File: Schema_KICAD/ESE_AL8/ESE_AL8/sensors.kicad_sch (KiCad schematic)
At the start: 27 parts, among them J201 JTAG/SWD, J202 Moteur1, J203 Moteur2, J204 LIDAR, J205 CB1, J206 CB2, J207 CB3, J208 CB4, SW201 SW_c/s, U201 ZXBM5210-SP, U202 ZXBM5210-SP, U203 ADXL343

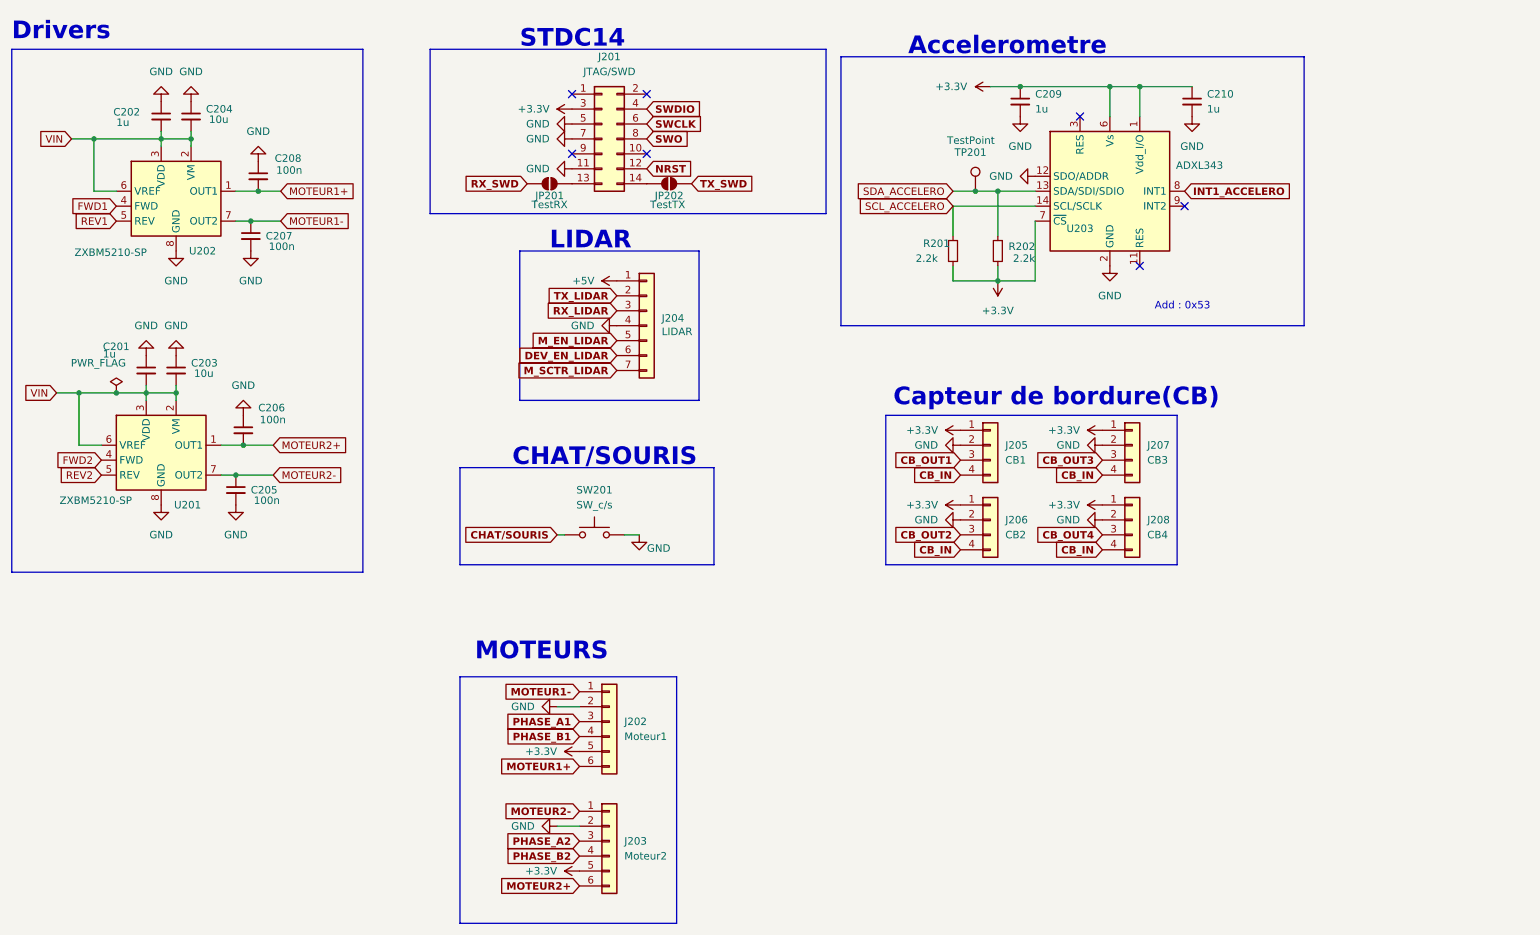
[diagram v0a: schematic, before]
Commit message: commit du code et kicad modifié
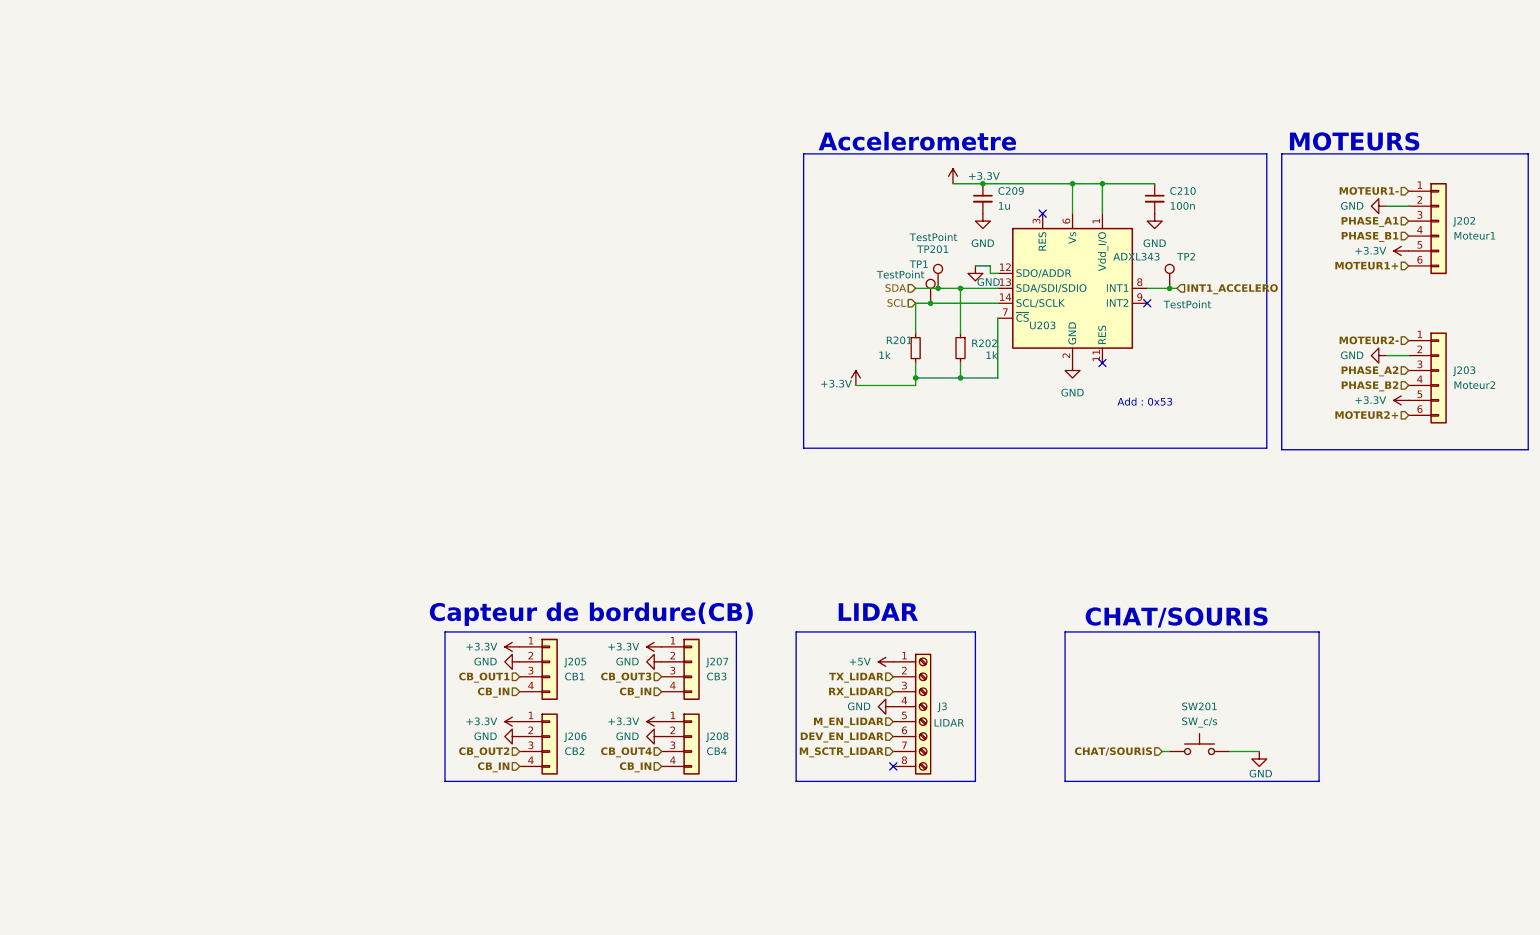
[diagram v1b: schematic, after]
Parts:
- removed C201, C202: 1u, Capacitor_SMD:C_0402_1005Metric_Pad0.74x0.62mm_HandSolder, symbol Device:C_Small
- removed C203, C204: 10u, Capacitor_SMD:C_0603_1608Metric_Pad1.08x0.95mm_HandSolder, symbol Device:C_Small
- removed C205, C206, C207, C208: 100n, Capacitor_SMD:C_0402_1005Metric_Pad0.74x0.62mm_HandSolder, symbol Device:C_Small
- removed J201: JTAG/SWD, Connector_PinHeader_1.27mm:PinHeader_2x07_P1.27mm_Vertical_SMD, symbol Connector_Generic:Conn_02x07_Odd_Even
- removed J204: LIDAR, Connector_JST:JST_EH_B7B-EH-A_1x07_P2.50mm_Vertical, symbol Connector_Generic:Conn_01x07
- removed JP201: TestRX, Jumper:SolderJumper-2_P1.3mm_Open_TrianglePad1.0x1.5mm, symbol Jumper:SolderJumper_2_Open
- removed JP202: TestTX, Jumper:SolderJumper-2_P1.3mm_Open_TrianglePad1.0x1.5mm, symbol Jumper:SolderJumper_2_Open
- removed U201, U202: ZXBM5210-SP, Package_SO:Diodes_SO-8EP, symbol Driver_Motor:ZXBM5210-SP
- added J3: LIDAR, symbol Connector:Screw_Terminal_01x08
- added TP1, TP2: TestPoint, TestPoint:TestPoint_Pad_D1.0mm, symbol Connector:TestPoint
- C210: value 1u -> 100n
- R201, R202: value 2.2k -> 1k
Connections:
- net +5V: now also J3.1 (Pin_1)
- net DEV_EN_LIDAR: now also J3.6 (Pin_6)
- net GND: now also J3.4 (Pin_4)
- net INT1_ACCELERO: now also TP2.1
- net M_EN_LIDAR: now also J3.5 (Pin_5)
- net M_SCTR_LIDAR: now also J3.7 (Pin_7)
- net RX_LIDAR: now also J3.3 (Pin_3)
- net TX_LIDAR: now also J3.2 (Pin_2)
- net SCL_ACCELERO renamed SCL
- net SCL: now also TP1.1
- net SDA_ACCELERO renamed SDA
- no-connect marks 7 -> 4
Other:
- note removed: "Drivers"
- note removed: "STDC14"
- moved on the sheet: C209, C210, J202, J203, J205, J206, J207, J208, R201, R202, SW201, TP201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
